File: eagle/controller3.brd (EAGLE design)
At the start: 97.5 x 48.2 mm, 24 parts, among them K1 SRD-05VDC-SL-C, K2 SRD-05VDC-SL-C, K3 SRD-05VDC-SL-C, T1 BC547, T2 BC547, T3 BC547, X1 VCC, X2 IN1, X3 IN2, X4 IN3

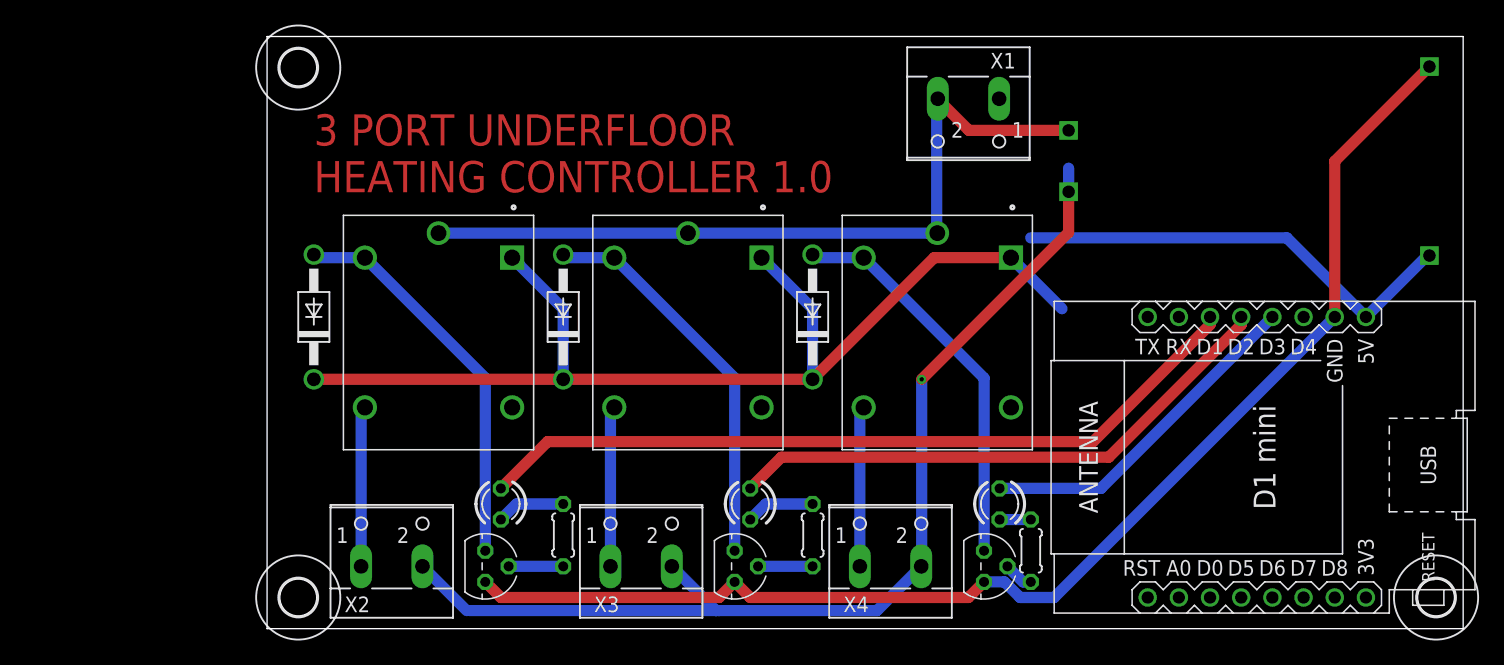
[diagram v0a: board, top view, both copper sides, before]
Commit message: Update to Version 1.1
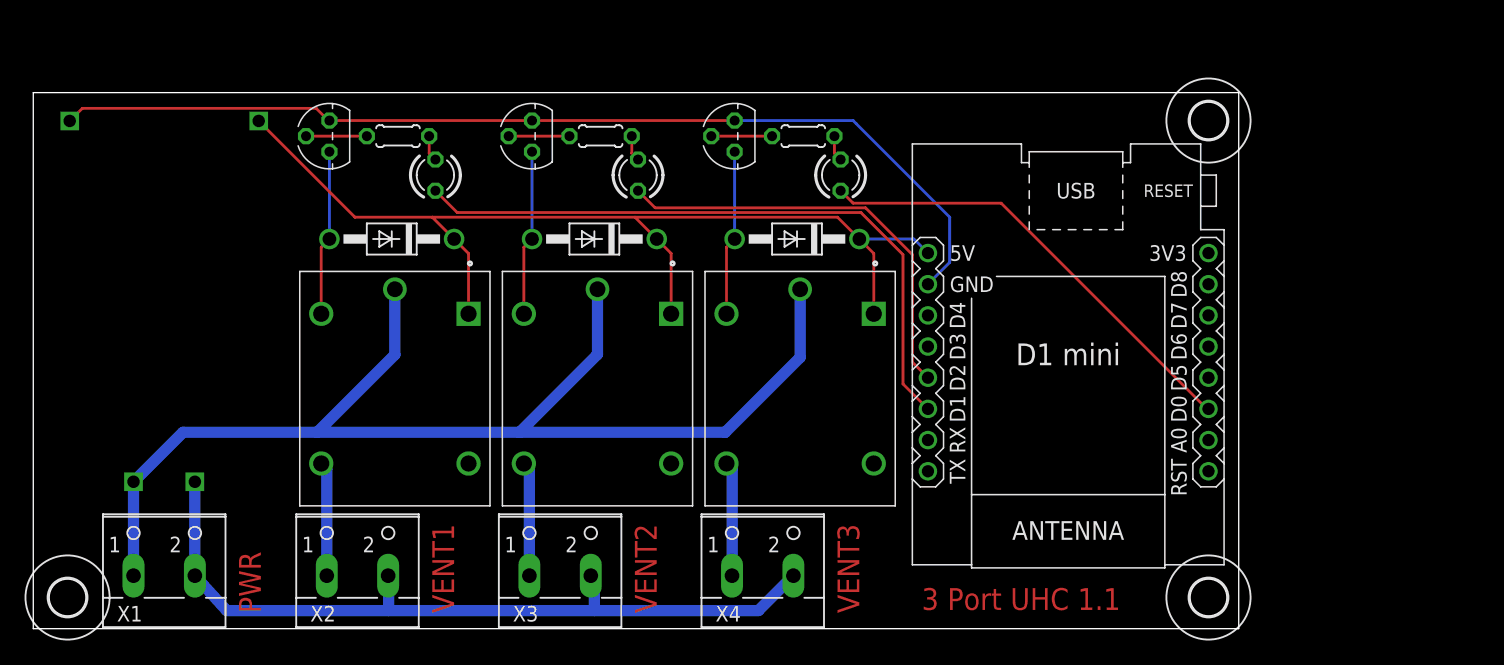
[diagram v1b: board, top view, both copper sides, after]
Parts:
- moved HLK1 89.1 mm to (10.7, 26.7), turned to 90 degrees
- moved U$2 85.8 mm to (95.8, 2.54)
- moved X1 74.9 mm to (10.7, 5.59), turned to 0 degrees
- moved U$4 43.1 mm to (95.8, 41.4)
- moved T3 40.5 mm to (57.1, 40.1), turned to 90 degrees
- moved T2 38.7 mm to (40.6, 40.1), turned to 90 degrees
- moved R3 38.5 mm to (62.7, 40.1), turned to 180 degrees
- moved T1 37.3 mm to (24.1, 40.1), turned to 90 degrees
- moved R2 36.8 mm to (46.2, 40.1), turned to 180 degrees
- moved R1 35.2 mm to (29.7, 40.1), turned to 180 degrees
- moved LED3 29.8 mm to (65.8, 37.0), turned to 90 degrees
- moved LED2 28.3 mm to (49.3, 37.0), turned to 90 degrees
- moved LED1 27.3 mm to (32.8, 37.0), turned to 90 degrees
- moved U$3 18.8 mm to (2.79, 2.54)
- moved U$1 18.1 mm to (84.3, 22.4), turned to 180 degrees
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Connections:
- removed net N$16: LED3.A, U$1.JP2.5
- new net N$17: LED3.A, U$1.JP1.3
- net 0V: now also X1.2; no longer X1.1
- net VCC: now also X1.1; no longer X1.2
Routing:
- net +5V: track 127.5 -> 84.3 mm
- net N$17: track 0.00 -> 37.3 mm
- net VCC: track 63.3 -> 100.3 mm
- net N$16: track 28.0 -> 0.00 mm
- net GND: track 104.9 -> 82.0 mm
- net 0V: track 86.2 -> 64.9 mm, vias 1 -> 0
- net N$4: track 32.2 -> 13.5 mm
- net N$3: track 32.2 -> 13.5 mm
- net N$1: track 32.2 -> 13.6 mm
- net N$14: track 46.2 -> 35.1 mm
- net N$15: track 63.9 -> 53.7 mm
- net N$12: track 13.1 -> 9.33 mm
- net N$2: track 13.1 -> 9.33 mm
- net N$11: track 13.1 -> 9.33 mm
- net N$20: track 5.61 -> 2.12 mm
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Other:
- board size 97.5 x 48.2 mm -> 98.2 x 43.7 mm
- board text added: "3 Port UHC 1.1"
- board text added: "PWR"
- board text added: "VENT1"
- board text added: "VENT2"
- board text added: "VENT3"
- board text removed: "3 PORT UNDERFLOOR HEATING CONTROLLER 1.0"
